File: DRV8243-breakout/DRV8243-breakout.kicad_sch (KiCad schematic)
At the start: 1 part, among them U1 PDRV8243HRXYQ1

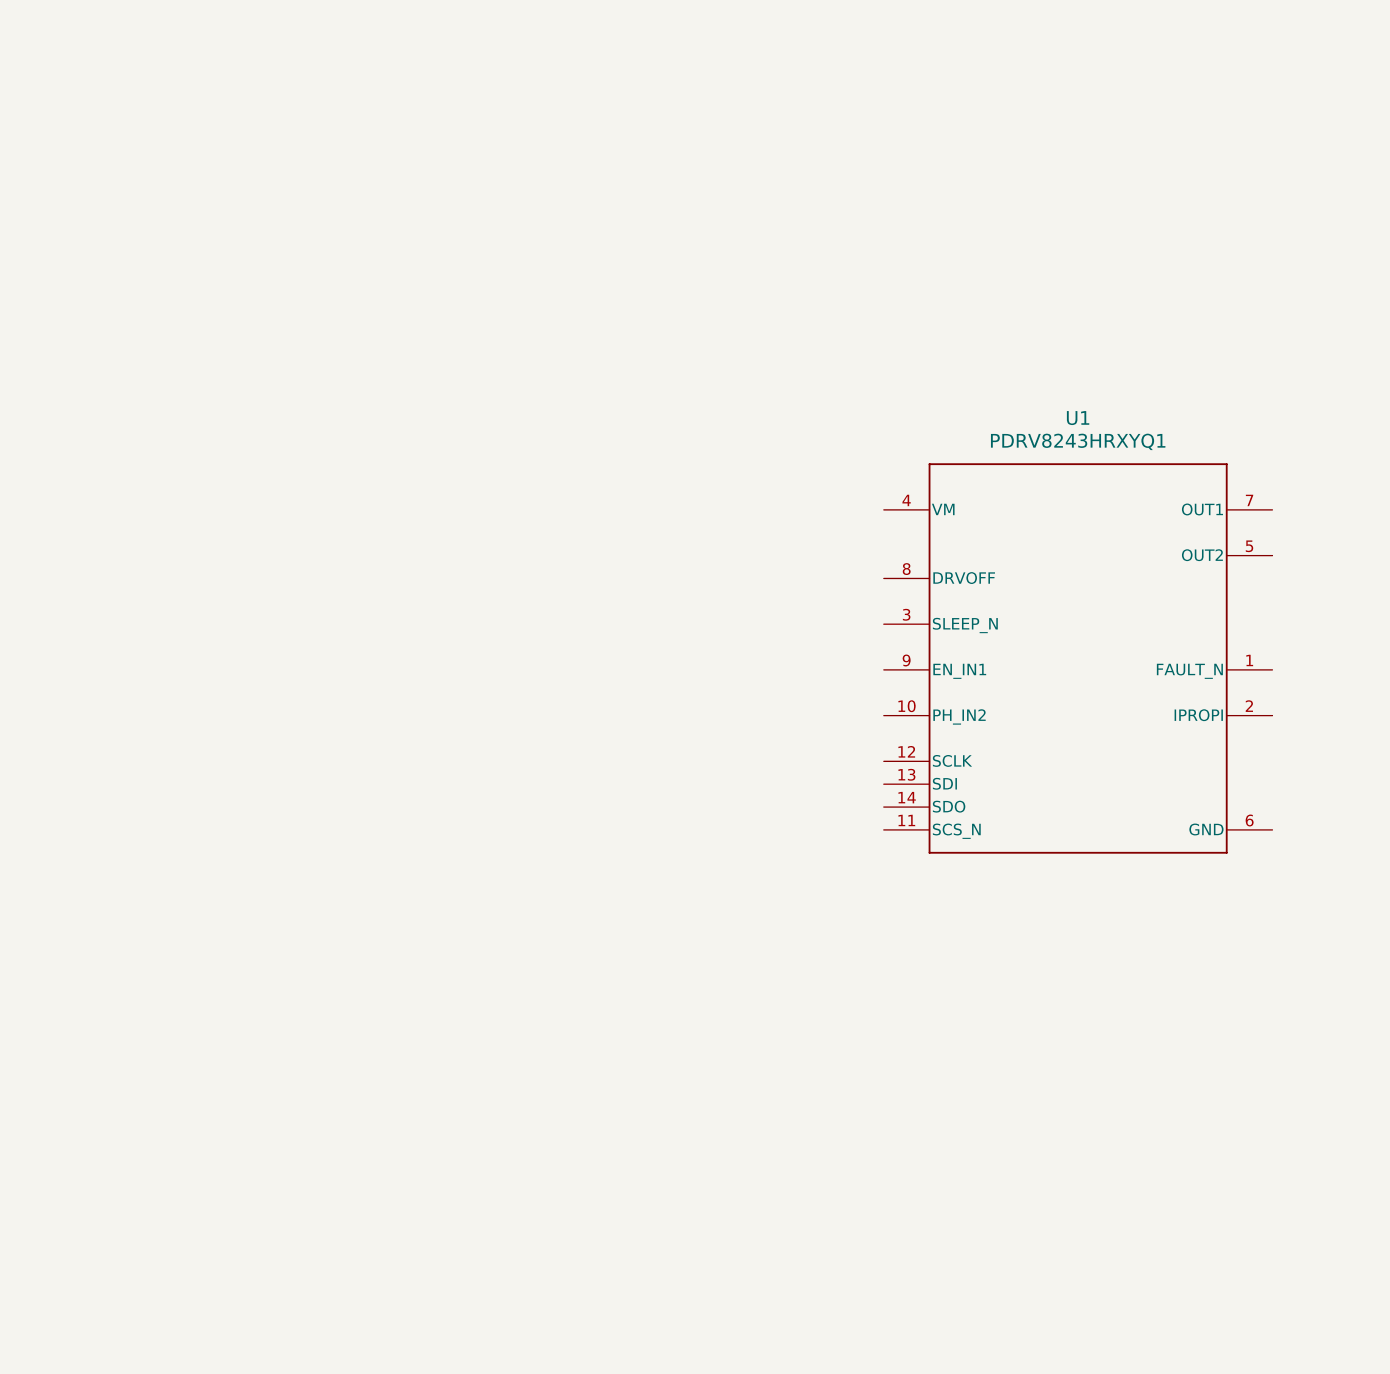
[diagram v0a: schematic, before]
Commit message: Minimal Setup
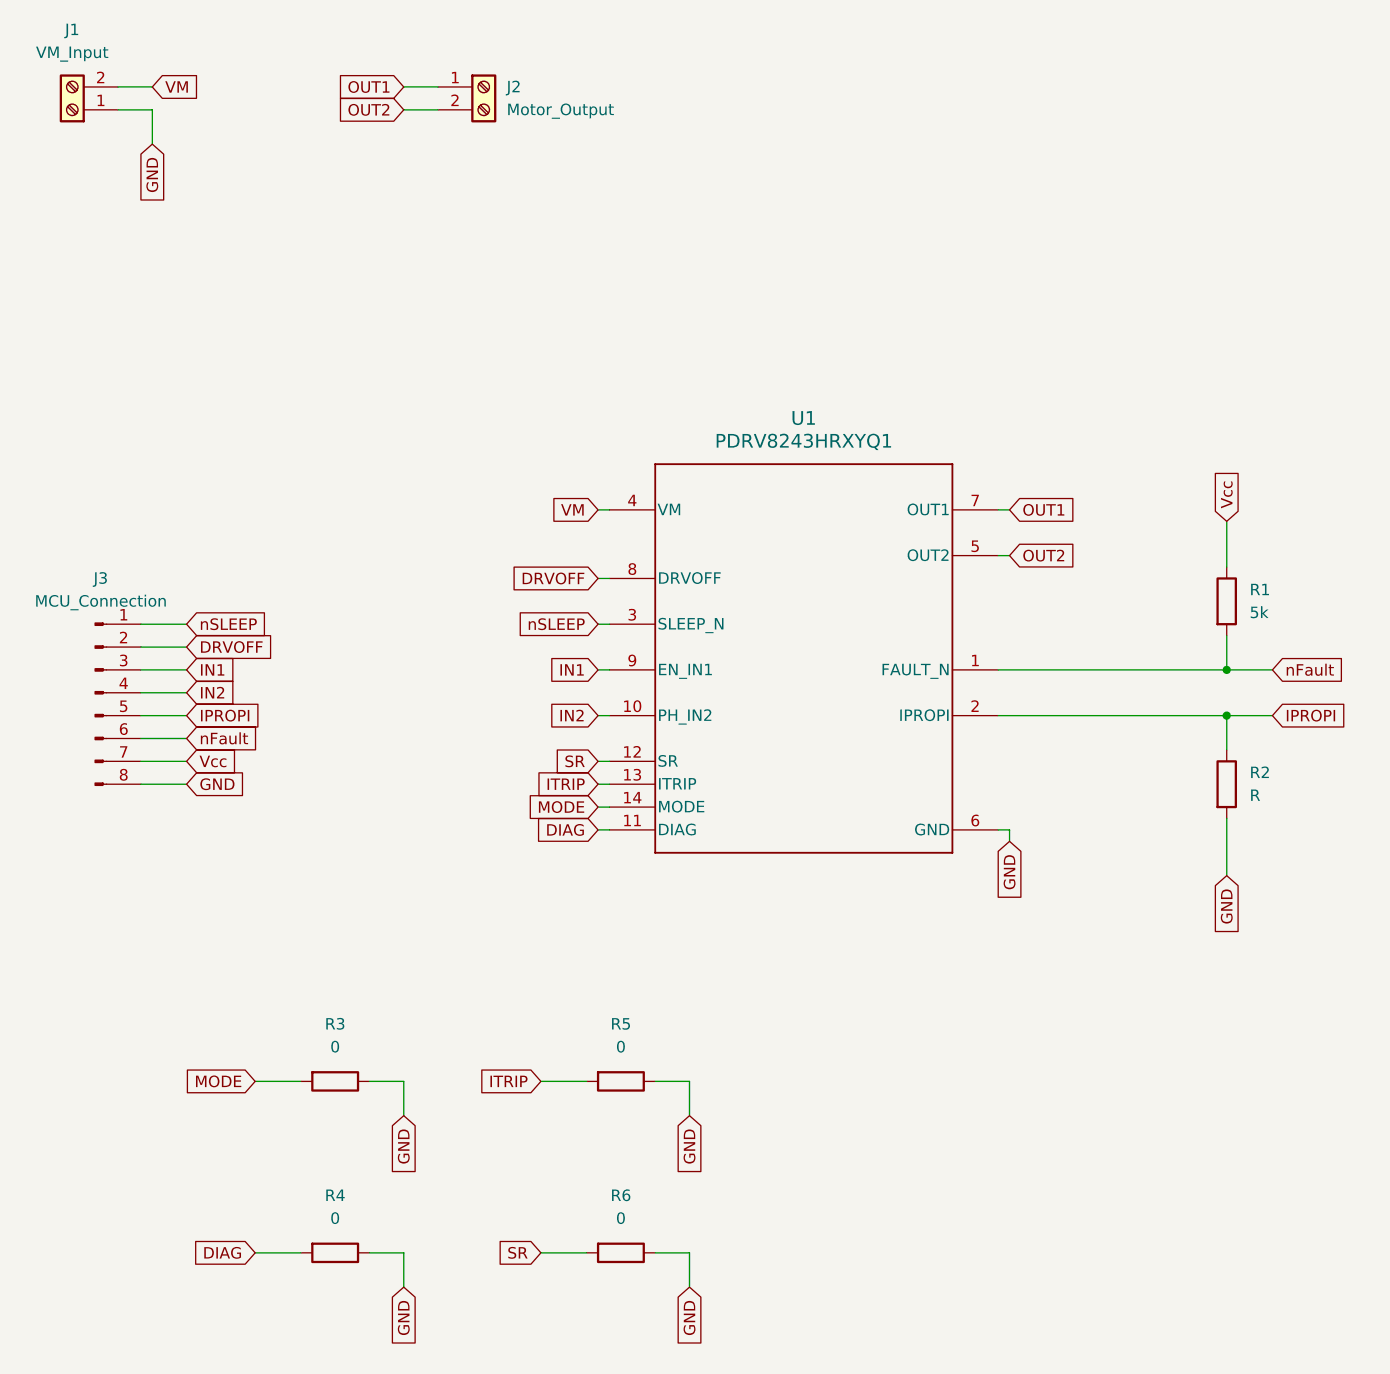
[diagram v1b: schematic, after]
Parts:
- added J1: VM_Input, symbol Connector:Screw_Terminal_01x02
- added J2: Motor_Output, symbol Connector:Screw_Terminal_01x02
- added J3: MCU_Connection, symbol Connector:Conn_01x08_Pin
- added R1: 5k, symbol Device:R
- added R2: R, symbol Device:R
- added R3, R4, R5, R6: 0, symbol Device:R
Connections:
- net nFault: now reaches U1.1 (FAULT_N)
- net nFault: now also J3.6 (Pin_6), R1.2
- net IN2: now reaches U1.10 (PH_IN2)
- net IN2: now also J3.4 (Pin_4)
- net DIAG: now reaches U1.11 (DIAG)
- net DIAG: now also R4.2
- net SR: now reaches U1.12 (SR)
- net SR: now also R6.2
- net ITRIP: now reaches U1.13 (ITRIP)
- net ITRIP: now also R5.2
- net MODE: now reaches U1.14 (MODE)
- net MODE: now also R3.2
- net IPROPI: now reaches U1.2 (IPROPI)
- net IPROPI: now also J3.5 (Pin_5), R2.1
- net nSLEEP: now reaches U1.3 (SLEEP_N)
- net nSLEEP: now also J3.1 (Pin_1)
- net VM: now reaches U1.4 (VM)
- net VM: now also J1.2 (Pin_2)
- net OUT2: now reaches U1.5 (OUT2)
- net OUT2: now also J2.2 (Pin_2)
- net GND: now reaches U1.6 (GND)
- net GND: now also J1.1 (Pin_1), J3.8 (Pin_8), R2.2, R3.1, R4.1, R5.1, R6.1
- net OUT1: now reaches U1.7 (OUT1)
- net OUT1: now also J2.1 (Pin_1)
- net DRVOFF: now reaches U1.8 (DRVOFF)
- net DRVOFF: now also J3.2 (Pin_2)
- net IN1: now reaches U1.9 (EN_IN1)
- net IN1: now also J3.3 (Pin_3)
- new net Vcc: J3.7 (Pin_7), R1.1
